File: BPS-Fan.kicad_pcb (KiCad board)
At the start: 2 copper layers, 43.6 x 42.8 mm, 25 parts, among them J1 LDRBRDConn, J2 FAN7, J3 FAN7, J4 FAN7, J5 FAN7, Q1 BUK9M23-80E, Q2 BUK9M23-80E, Q4 BUK9M23-80E, Q5 BUK9M23-80E

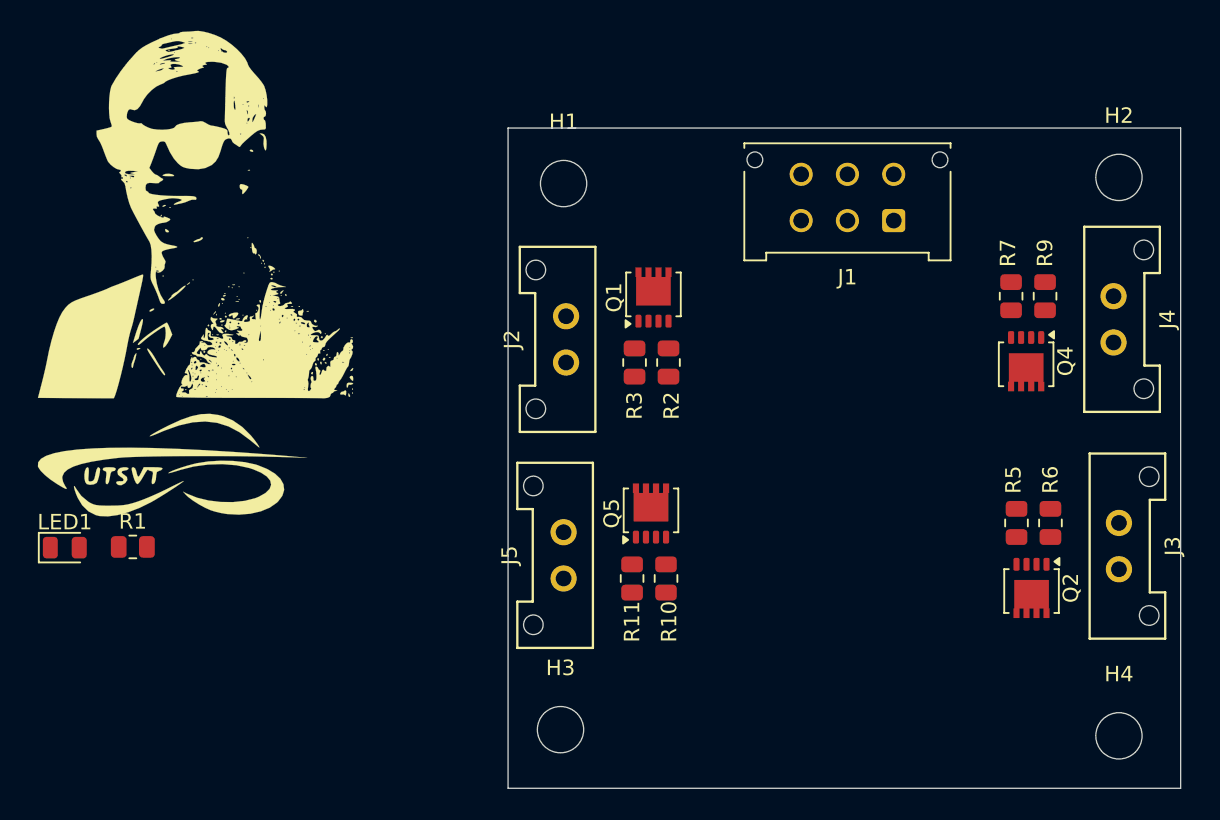
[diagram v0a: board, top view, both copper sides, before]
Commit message: layout go brrr
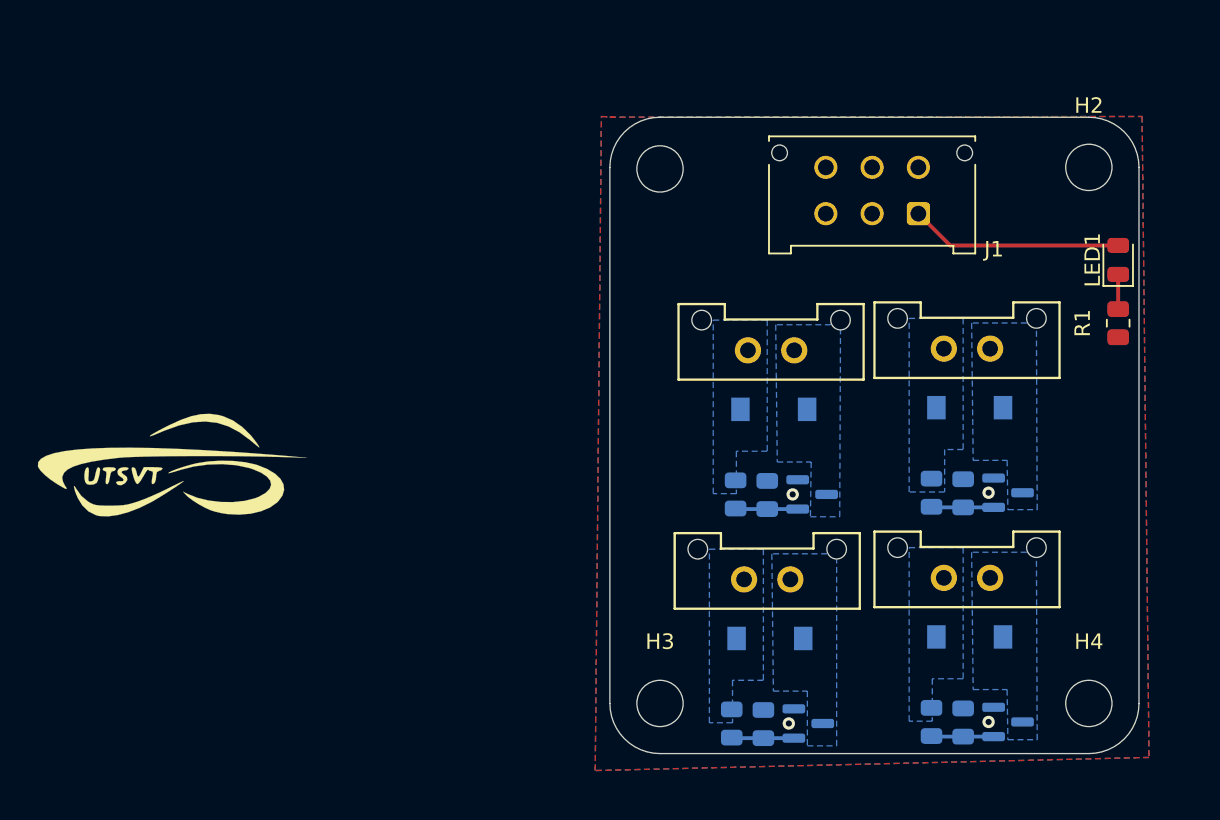
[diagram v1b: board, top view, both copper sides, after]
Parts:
- removed Q1, Q2, Q4, Q5: BUK9M23-80E, Package_TO_SOT_SMD:LFPAK33
- added D1: VSSAF522-M3/H, UTSVT_Passive:DO-221AC, B.Cu at (144.2, 91.5)
- added D2: VSSAF522-M3/H, UTSVT_Passive:DO-221AC, B.Cu at (131.5, 76.8)
- added D4: VSSAF522-M3/H, UTSVT_Passive:DO-221AC, B.Cu at (144.2, 76.6)
- added D5: VSSAF522-M3/H, UTSVT_Passive:DO-221AC, B.Cu at (131.3, 91.6)
- added Q3: IRLML0030, Package_TO_SOT_SMD:SOT-23, B.Cu at (146.7, 97.0)
- added Q6: IRLML0030, Package_TO_SOT_SMD:SOT-23, B.Cu at (134.0, 82.3)
- added Q7: IRLML0030, Package_TO_SOT_SMD:SOT-23, B.Cu at (146.7, 82.2)
- added Q8: IRLML0030, Package_TO_SOT_SMD:SOT-23, B.Cu at (133.8, 97.1)
- LOGO1, R10, R11, R2, R3, R5, R6, R7, R9: moved to B.Cu
- moved LOGO1 79.4 mm to (171.2, 78.5), turned to 180 degrees
- moved LED1 70.8 mm to (153.8, 67.1), turned to 90 degrees
- moved R1 65.5 mm to (153.8, 71.2), turned to -90 degrees
- moved R3 31.6 mm to (143.8, 97.1), turned to 90 degrees
- moved R2 28.9 mm to (141.7, 97.0), turned to -90 degrees
- moved J2 28.2 mm to (142.5, 87.7), turned to 0 degrees
- moved J3 26.5 mm to (129.8, 72.9), turned to 0 degrees
- moved R6 18.4 mm to (131.1, 82.3)
- moved R5 18.3 mm to (129.0, 82.3)
- moved R9 13.8 mm to (143.8, 82.2)
- moved R7 13.7 mm to (141.7, 82.2)
- moved R11 12.7 mm to (130.8, 97.2), turned to 90 degrees
- moved J5 11.7 mm to (129.6, 87.8), turned to 0 degrees
- moved J4 11.5 mm to (142.5, 72.8), turned to 0 degrees
- moved R10 10.3 mm to (128.8, 97.1), turned to -90 degrees
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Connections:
- J2 pad 2: Net-(D1-A) -> /Driver1/FAN-
- J3 pad 2: Net-(D2-A) -> /Driver2/FAN-
- J4 pad 2: Net-(D4-A) -> /Driver3/FAN-
- J5 pad 2: Net-(D5-A) -> /Driver4/FAN-
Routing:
- net +12V: track 0.00 -> 13.8 mm
- net /FAN4_BPS: track 0.00 -> 4.04 mm
- net /FAN2_BPS: track 0.00 -> 4.04 mm
- net /FAN1_BPS: track 0.00 -> 4.04 mm
- net /FAN3_BPS: track 0.00 -> 4.04 mm
- net Net-(LED1-K): track 0.00 -> 2.25 mm
- net GNDPWR: vias 0 -> 4
- added copper zone on B.Cu, net +12V
- added copper zone on B.Cu, net /Driver1/FAN-
- added copper zone on B.Cu, net /Driver2/FAN-
- added copper zone on B.Cu, net /Driver3/FAN-
- added copper zone on B.Cu, net /Driver4/FAN-
- added copper zone on B.Cu, net GNDPWR
- added copper zone on F.Cu, net GNDPWR
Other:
- board size 43.6 x 42.8 mm -> 34.3 x 41.2 mm
